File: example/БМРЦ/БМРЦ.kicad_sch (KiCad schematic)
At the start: 59 parts

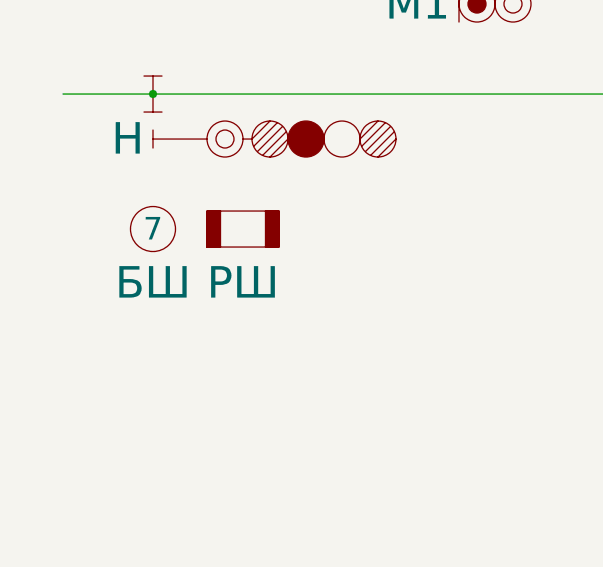
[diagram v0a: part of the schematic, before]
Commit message: Обновлены РШ и БШ
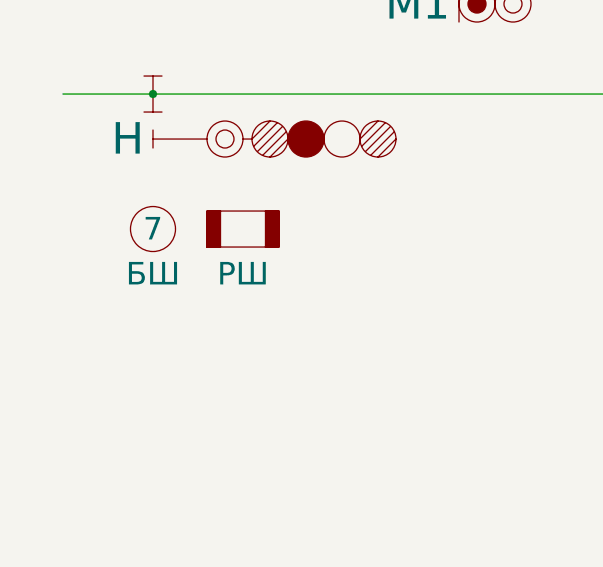
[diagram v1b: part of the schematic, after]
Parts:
- БШ1: Ордината (none) -> (720); Тип (none) -> ШМБ-У
- РШ1: Ордината (none) -> (720); Тип (none) -> ШРУ-М
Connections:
- new net: Изостык11. (привязка), Стрелка5.1, Стрелка6.1
- new net: Изостык14. (привязка), Стрелка6.1, Стрелка7.1
- new net: Изостык9. (привязка), Стрелка3.1, Стрелка5.1
- new net: Изостык12. (привязка), Стрелка4.1, Стрелка6.1
- new net: Изостык7. (привязка), Стрелка3.1, Стрелка4.1
- new net: Изостык8. (привязка), Стрелка1.1, Стрелка2.1
- new net: Изостык10. (привязка), Стрелка2.1, Стрелка8.1
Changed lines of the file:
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@@
 		)
 		(property "Шкаф" "РШ"
-			(at 50 226 0)
-			(do_not_autoplace yes)
-			(effects
-				(font
-					(size 3.5 3.5)
-				)
+			(at 50 225 0)
+			(do_not_autoplace yes)
+			(effects
+				(font
+					(size 2.5 2.5)
+				)
+			)
+		)
+		(property "Ордината" "(720)"
+			(at 50 211 0)
+			(effects
+				(font
+					(size 2.5 2.5)
+				)
+				(hide yes)
+			)
+		)
+		(property "Тип" "ШРУ-М"
+			(at 50 215 0)
+			(effects
+				(font
+					(size 2.5 2.5)
+				)
+				(hide yes)
 			)
 		)
@@
 		)
 		(property "Шкаф" "БШ"
-			(at 40 226 0)
-			(do_not_autoplace yes)
-			(effects
-				(font
-					(size 3.5 3.5)
-				)
-			)
-		)
+			(at 40 225 0)
+			(do_not_autoplace yes)
+			(effects
+				(font
+					(size 2.5 2.5)
+				)
+			)
+		)
+		(property "Ордината" "(720)"
+			(at 40 215 0)
+			(effects
+				(font
+					(size 2.5 2.5)
+				)
+				(hide yes)
+			)
+		)
+		(property "Тип" "ШМБ-У"
+			(at 40 210 0)
+			(effects
+				(font
+					(size 2.5 2.5)
+				)
+				(hide yes)
+			)
+		)

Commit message: Упрощены УГО ДТ для фазочувствительных РЦ, скрыты точки для двойных СС
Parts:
- Входной1: now left out of the parts list
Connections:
- new net: Изостык11. (привязка), Стрелка5.1, Стрелка6.1
- new net: Изостык14. (привязка), Стрелка6.1, Стрелка7.1
- new net: Изостык9. (привязка), Стрелка3.1, Стрелка5.1
- new net: Изостык12. (привязка), Стрелка4.1, Стрелка6.1
- new net: Изостык7. (привязка), Стрелка3.1, Стрелка4.1
- new net: Изостык8. (привязка), Стрелка1.1, Стрелка2.1
- new net: Изостык10. (привязка), Стрелка2.1, Стрелка8.1
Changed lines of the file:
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@@
 	)
 	(symbol
+		(lib_name "SCB:Изостык")
 		(lib_id "SCB:Изостык")
 		(at 330 160 0)
@@
 	)
 	(symbol
+		(lib_name "SCB:Изостык")
 		(lib_id "SCB:Изостык")
 		(at 208 190 0)
@@
 	)
 	(symbol
+		(lib_name "SCB:Стрелка_спаренная")
 		(lib_id "SCB:Стрелка_спаренная")
 		(at 284 175 0)
@@
 	)
 	(symbol
+		(lib_name "SCB:Изостык")
 		(lib_id "SCB:Изостык")
 		(at 157 175 0)
@@
 	)
 	(symbol
+		(lib_name "SCB:Изостык")
 		(lib_id "SCB:Изостык")
 		(at 334 130 0)
@@
 	)
 	(symbol
+		(lib_name "SCB:Изостык")
 		(lib_id "SCB:Изостык")
 		(at 226 175 0)
@@
 	)
 	(symbol
+		(lib_name "SCB:Изостык")
 		(lib_id "SCB:Изостык")
 		(at 350 220 0)
@@
 	)
 	(symbol
+		(lib_name "SCB:Изостык")
 		(lib_id "SCB:Изостык")
 		(at 86 160 0)
@@
 	)
 	(symbol
+		(lib_name "SCB:Изостык")
 		(lib_id "SCB:Изостык")
 		(at 279 175 0)
@@
 		(mirror y)
 		(unit 2)
-		(exclude_from_sim no)
-		(in_bom yes)
-		(on_board yes)
+		(exclude_from_sim yes)
+		(in_bom no)
+		(on_board no)
 		(dnp no)
 		(fields_autoplaced yes)
@@
 	)
 	(symbol
+		(lib_name "SCB:Стрелка_спаренная_15")
 		(lib_id "SCB:Стрелка_спаренная_15")
 		(at 148 175 0)
@@
 	)
 	(symbol
+		(lib_name "SCB:Изостык")
 		(lib_id "SCB:Изостык")
 		(at 313 175 0)
@@
 	)
 	(symbol
+		(lib_name "SCB:Стрелка_спаренная_15")
 		(lib_id "SCB:Стрелка_спаренная_15")
 		(at 127 205 0)
@@
 	)
 	(symbol
+		(lib_name "SCB:Изостык")
 		(lib_id "SCB:Изостык")
 		(at 74 190 0)
@@
 	)
 	(symbol
+		(lib_name "SCB:Изостык")
 		(lib_id "SCB:Изостык")
 		(at 249 160 0)
@@
 	)
 	(symbol
+		(lib_name "SCB:Изостык")
 		(lib_id "SCB:Изостык")
 		(at 132 190 0)
@@
 	)
 	(symbol
+		(lib_name "SCB:Изостык")
 		(lib_id "SCB:Изостык")
 		(at 167 205 0)
@@
 	)
 	(symbol
+		(lib_name "SCB:Изостык")
 		(lib_id "SCB:Изостык")
 		(at 350 205 0)
@@
 	)
 	(symbol
+		(lib_name "SCB:Изостык")
 		(lib_id "SCB:Изостык")
 		(at 40 190 0)
@@
 	)
 	(symbol
+		(lib_name "SCB:Изостык")
 		(lib_id "SCB:Изостык")
 		(at 40 205 0)
@@
 	)
 	(symbol
+		(lib_name "SCB:Стрелка_спаренная_15")
 		(lib_id "SCB:Стрелка_спаренная_15")
 		(at 294 205 0)
@@
 	)
 	(symbol
+		(lib_name "SCB:Изостык")
 		(lib_id "SCB:Изостык")
 		(at 375 160 0)
@@
 	)
 	(symbol
+		(lib_name "SCB:Изостык")
 		(lib_id "SCB:Изостык")
 		(at 82 175 0)
@@
 	)
 	(symbol
+		(lib_name "SCB:Стрелка_спаренная_15")
 		(lib_id "SCB:Стрелка_спаренная_15")
 		(at 190 175 0)
@@
 	)
 	(symbol
+		(lib_name "SCB:Стрелка_спаренная_15")
 		(lib_id "SCB:Стрелка_спаренная_15")
 		(at 79 190 0)
@@
 	)
 	(symbol
+		(lib_name "SCB:Изостык")
 		(lib_id "SCB:Изостык")
 		(at 123 205 0)
@@
 	)
 	(symbol
+		(lib_name "SCB:Изостык")
 		(lib_id "SCB:Изостык")
 		(at 307 205 0)
@@
 		(at 40 210 180)
 		(unit 1)
-		(exclude_from_sim no)
-		(in_bom yes)
-		(on_board yes)
+		(exclude_from_sim yes)
+		(in_bom no)
+		(on_board no)
 		(dnp no)
 		(fields_autoplaced yes)
@@
 	)
 	(symbol
+		(lib_name "SCB:Изостык")
 		(lib_id "SCB:Изостык")
 		(at 128 160 0)
@@
 	)
 	(symbol
+		(lib_name "SCB:Изостык")
 		(lib_id "SCB:Изостык")
 		(at 286 190 0)
@@
 	)
 	(symbol
+		(lib_name "SCB:Изостык")
 		(lib_id "SCB:Изостык")
 		(at 290 160 0)
